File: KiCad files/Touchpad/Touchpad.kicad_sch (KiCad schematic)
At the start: 18 parts, among them J1 Conn_02x03_Counter_Clockwise, J2 Conn_02x03_Counter_Clockwise, J3 Conn_01x07_Male, U1 TTP223-BA6, U2 TTP223-BA6, U3 TTP223-BA6

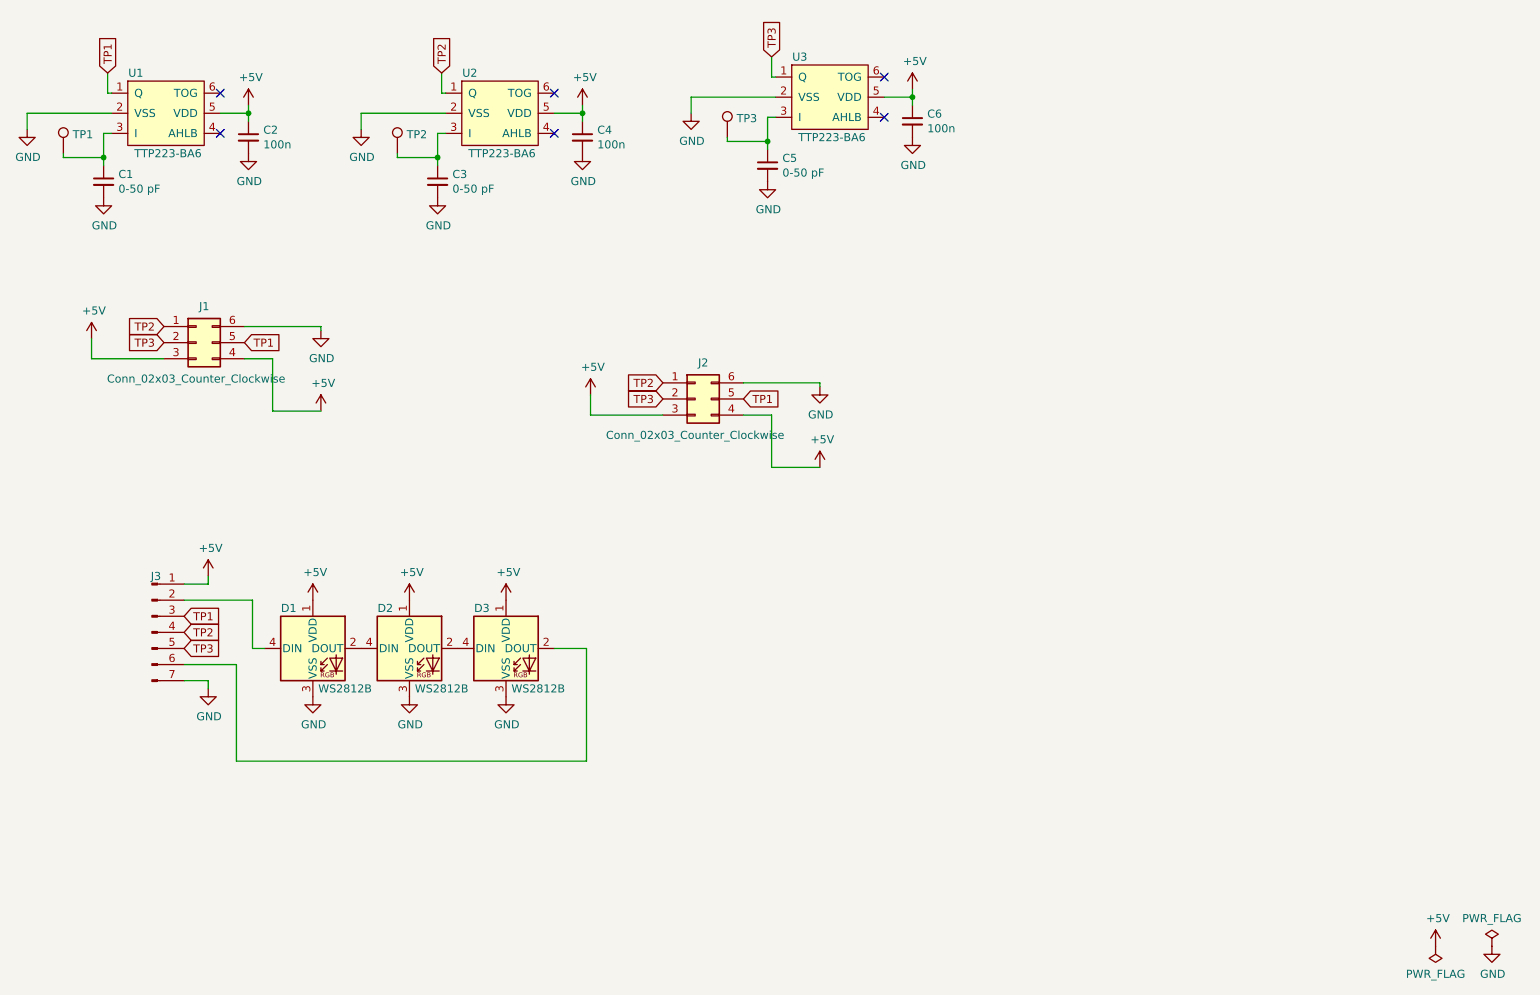
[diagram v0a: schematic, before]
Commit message: update
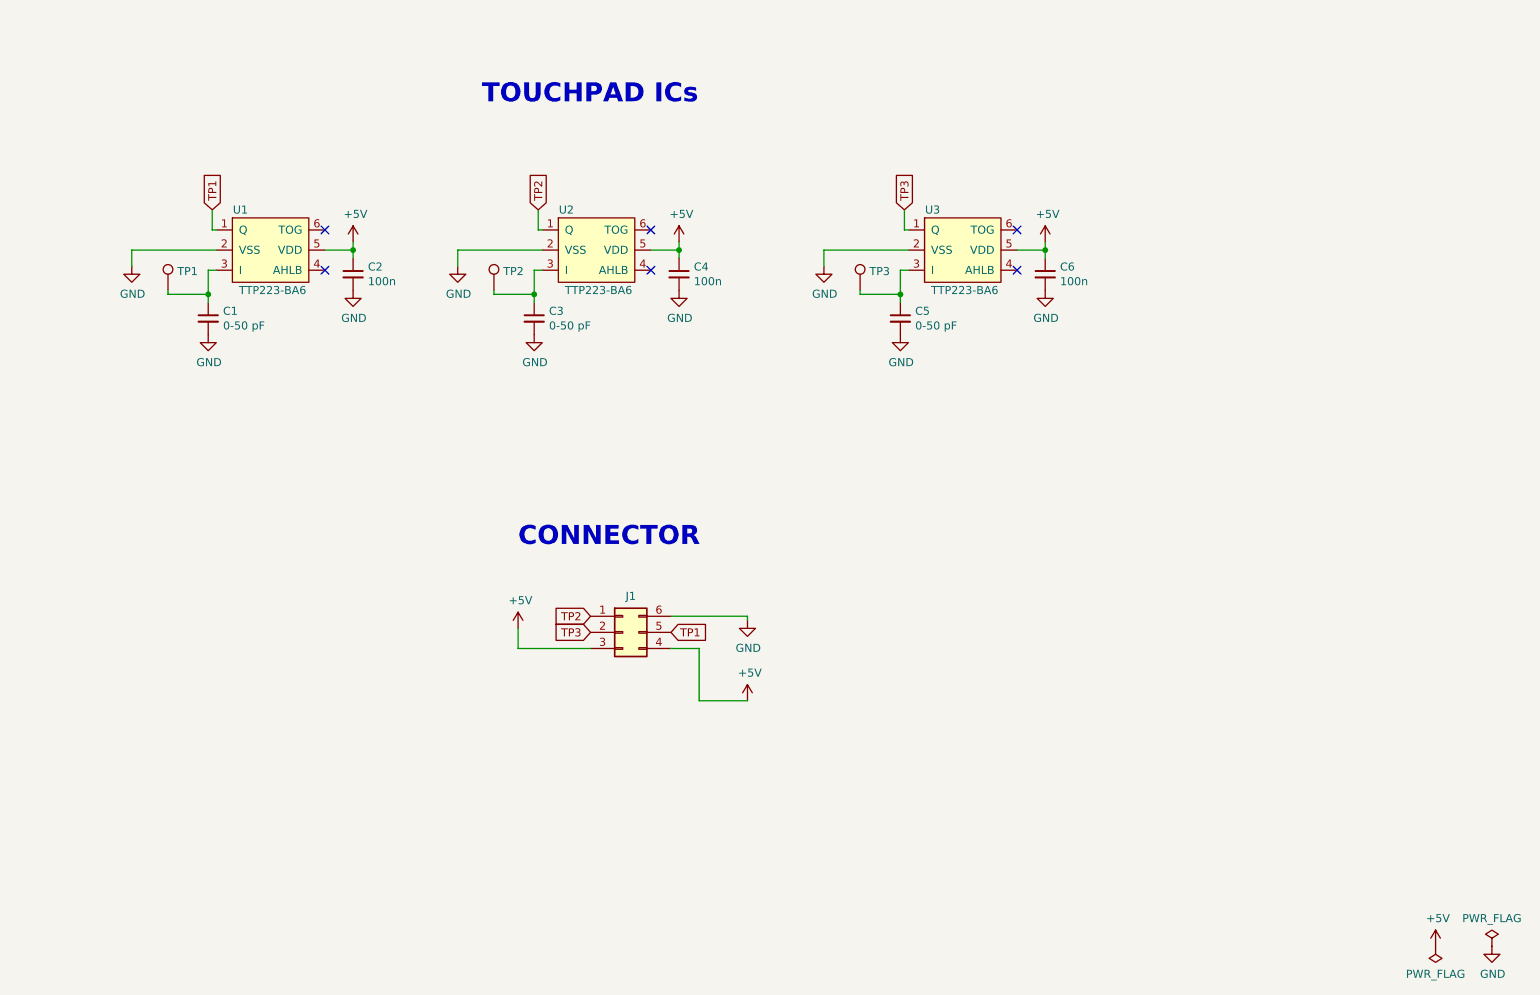
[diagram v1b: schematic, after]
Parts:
- removed D1, D2, D3: WS2812B, LED_SMD:LED_WS2812B_PLCC4_5.0x5.0mm_P3.2mm, symbol LED:WS2812B
- removed J2: Conn_02x03_Counter_Clockwise, Connector_PinHeader_1.27mm:PinHeader_2x03_P1.27mm_Vertical, symbol Connector_Generic:Conn_02x03_Counter_Clockwise
- removed J3: Conn_01x07_Male, Connector_PinHeader_2.54mm:PinHeader_1x07_P2.54mm_Vertical, symbol Connector:Conn_01x07_Male
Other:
- note added: "CONNECTOR"
- note added: "TOUCHPAD ICs"
- moved on the sheet: C1, C2, C3, C4, C5, C6, J1, TP1, TP2, TP3, U1, U2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
